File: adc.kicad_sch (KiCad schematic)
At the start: 87 parts, among them U35 MCP6004, U36 MCP6004, U46 MCP6004, U8 MCP6004

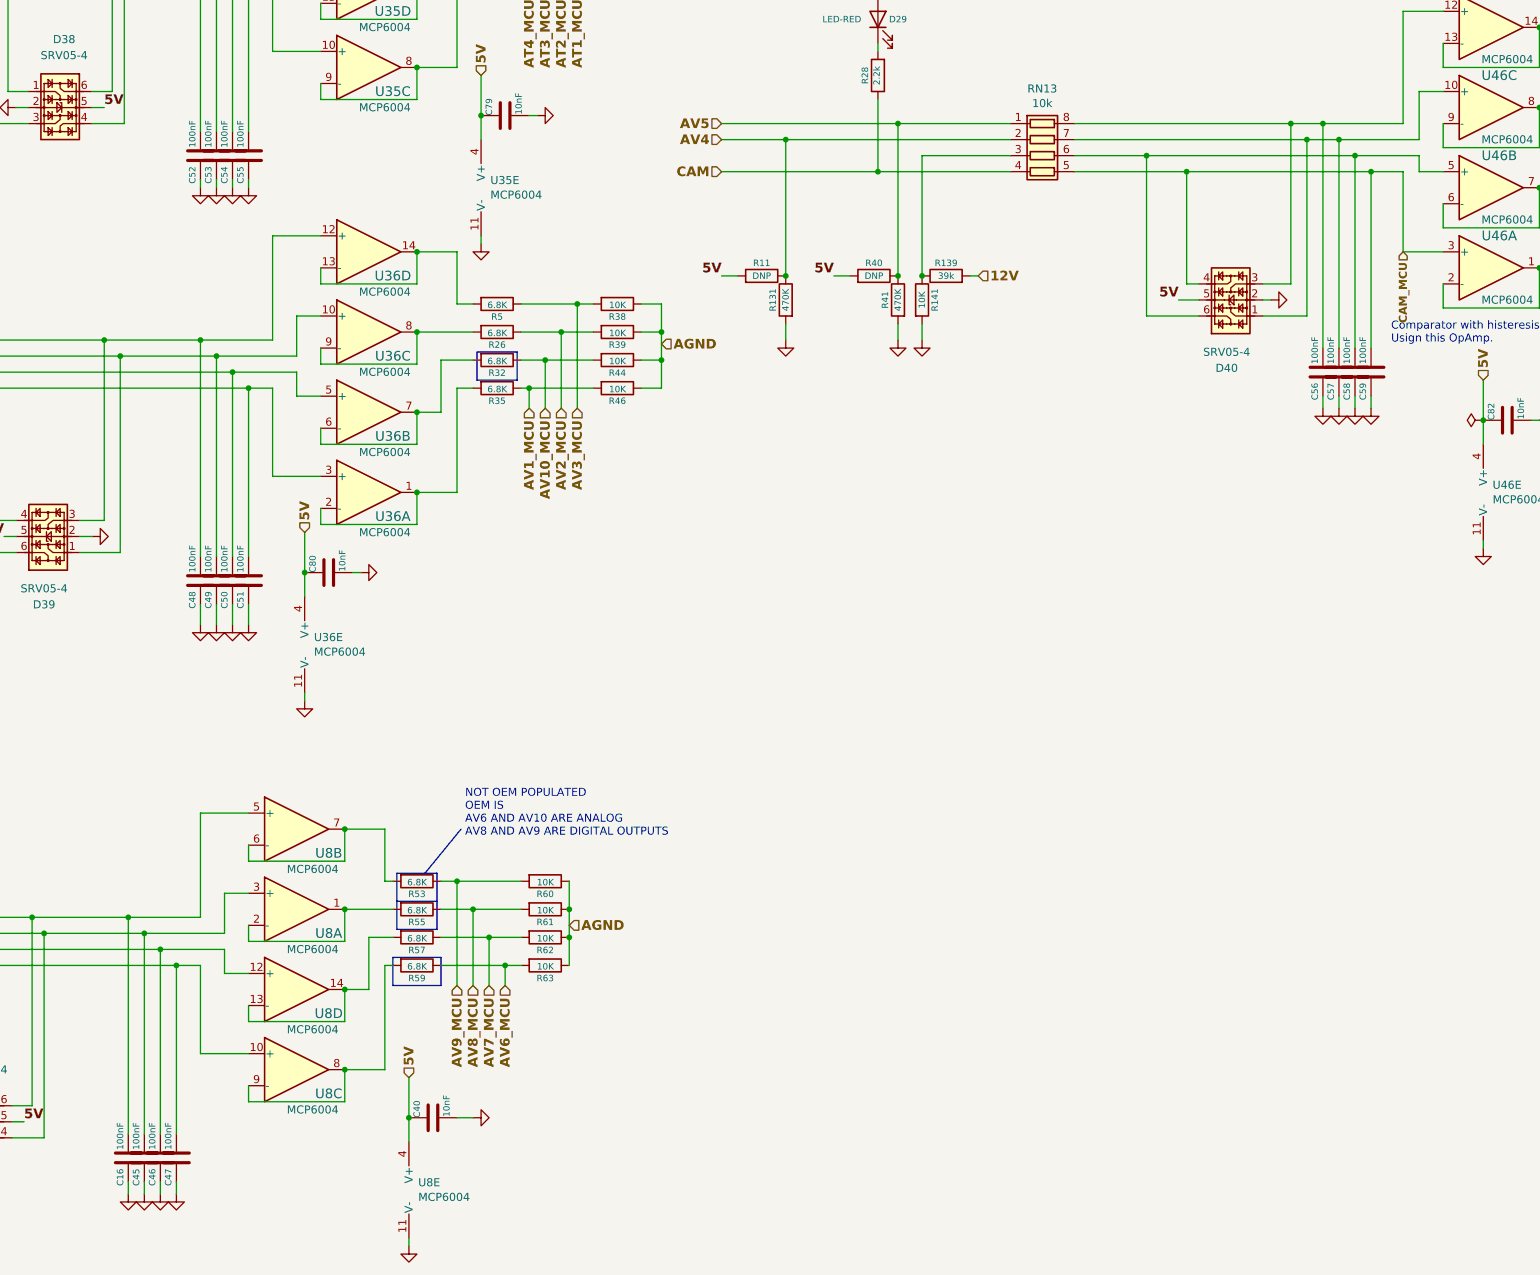
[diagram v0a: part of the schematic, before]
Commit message: KiCAD6 version
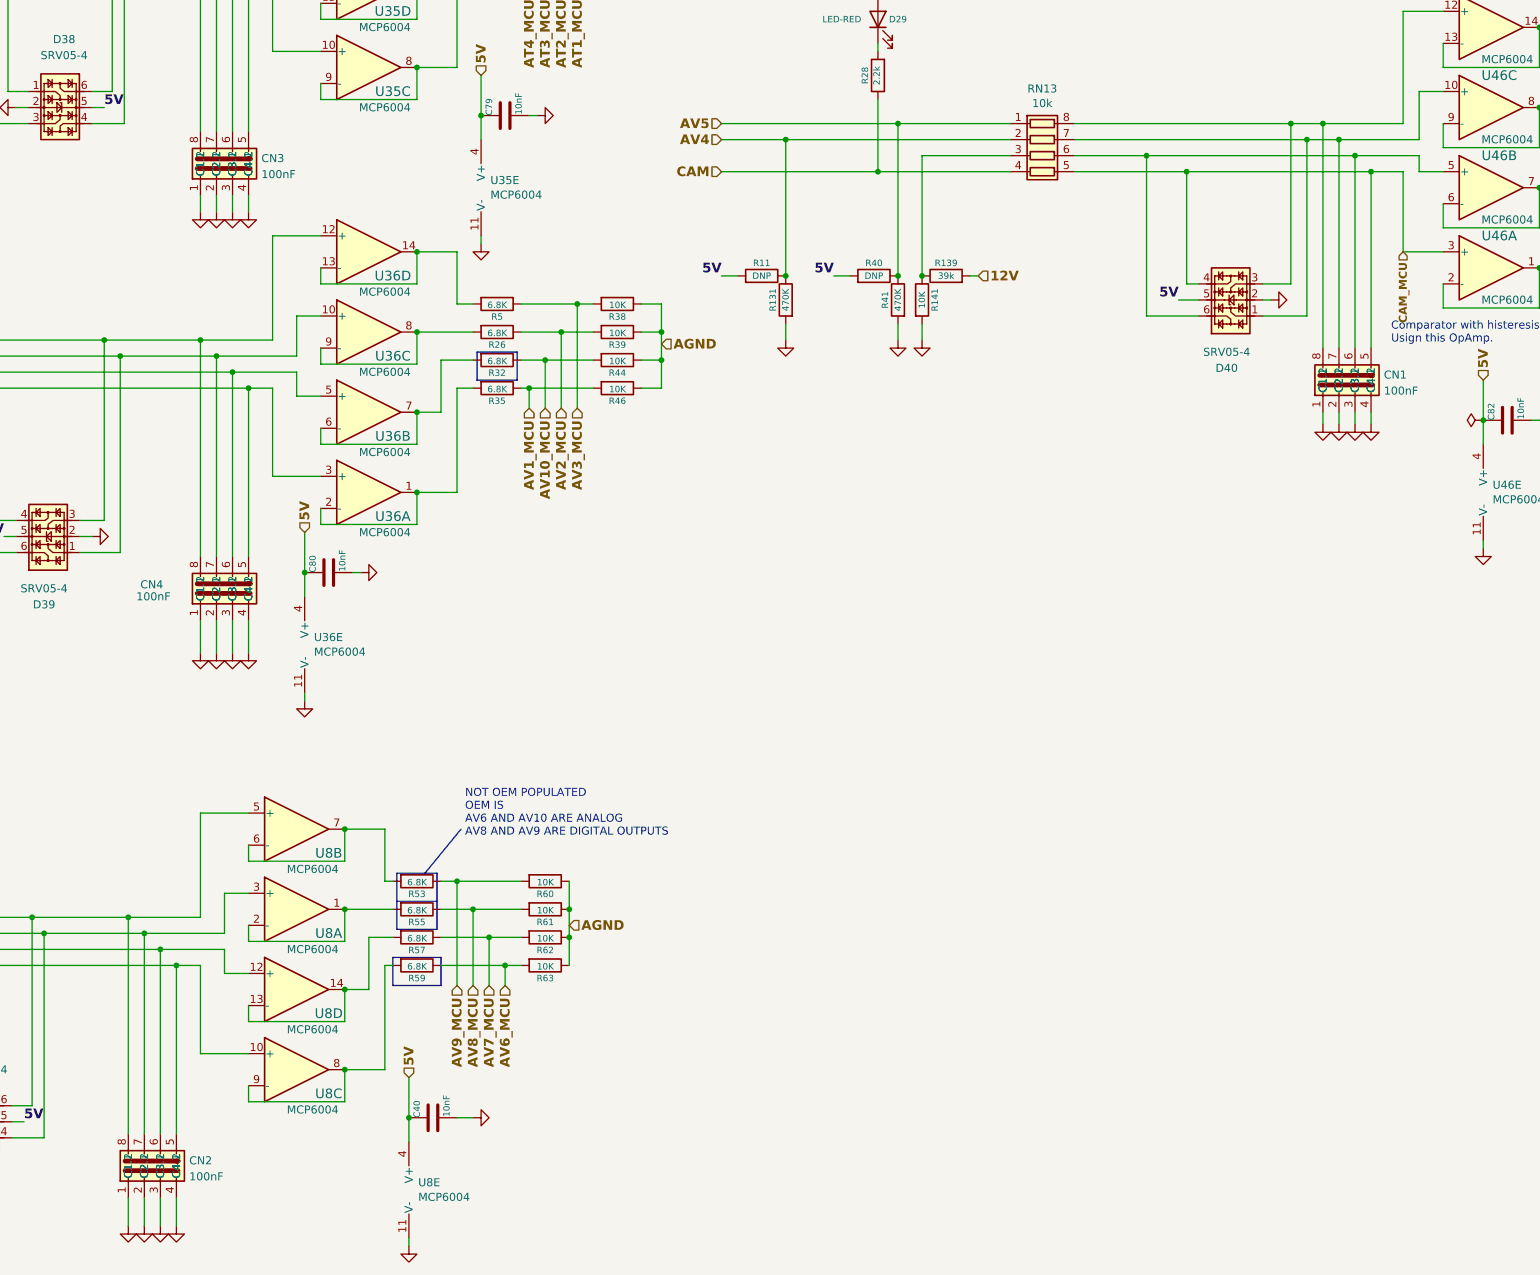
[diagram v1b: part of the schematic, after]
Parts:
- removed C16, C45, C46, C47, C48, C49, C50, C51, C52, C53, C54, C55, C56, C57, C58, C59: 100nF, Capacitor_SMD:C_0402_1005Metric, symbol Device:C
- added CN1, CN2, CN3, CN4: 100nF, Resistor_SMD:R_Array_Convex_4x0603, symbol rusefi_caparray:CN_Pack04
- R131, R24, R31, R34, R37, R41, R52, R54, R56, R58: footprint Resistor_SMD:R_0402_1005Metric -> Resistor_SMD:R_0603_1608Metric
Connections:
- net CAM_MCU: now also CN1.5 (C4.2)
- net GND: now also CN1.1 (C1.1), CN1.2 (C2.1), CN1.3 (C3.1), CN1.4 (C4.1), CN2.1 (C1.1), CN2.2 (C2.1), CN2.3 (C3.1), CN2.4 (C4.1), CN3.1 (C1.1), CN3.2 (C2.1), CN3.3 (C3.1), CN3.4 (C4.1), CN4.1 (C1.1), CN4.2 (C2.1), CN4.3 (C3.1), CN4.4 (C4.1)
- net at D38.3, RN3.6 (R3.2), U35.12 (+): now also CN3.6 (C3.2)
- net at D38.1, RN3.5 (R4.2), U35.10 (+): now also CN3.5 (C4.2)
- net at D38.6, RN3.8 (R1.2), U35.5 (+): now also CN3.8 (C1.2)
- net at D38.4, RN3.7 (R2.2), U35.3 (+): now also CN3.7 (C2.2)
- net at D13.3, RN2.6 (R3.2), U8.12 (+): now also CN2.6 (C3.2)
- net at D13.1, RN2.5 (R4.2), U8.10 (+): now also CN2.5 (C4.2)
- net at D13.6, RN2.8 (R1.2), U8.5 (+): now also CN2.8 (C1.2)
- net at D13.4, RN2.7 (R2.2), U8.3 (+): now also CN2.7 (C2.2)
- net at D39.3, RN4.8 (R1.2), U36.12 (+): now also CN4.8 (C1.2)
- net at D39.1, RN4.7 (R2.2), U36.10 (+): now also CN4.7 (C2.2)
- net at D39.6, RN4.6 (R3.2), U36.5 (+): now also CN4.6 (C3.2)
- net at D39.4, RN4.5 (R4.2), U36.3 (+): now also CN4.5 (C4.2)
- net at D40.3, RN13.8 (R1.2), U46.12 (+): now also CN1.8 (C1.2)
- net at D40.1, RN13.7 (R2.2), U46.10 (+): now also CN1.7 (C2.2)
- net at D40.6, RN13.6 (R3.2), U46.5 (+): now also CN1.6 (C3.2)
